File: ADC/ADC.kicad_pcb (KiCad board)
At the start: 2 copper layers, 38.1 x 63.5 mm, 98 parts, among them P1 CONN_02X05, P2 CONN_02X08, U1 MICA, U2 MICB, U3 TL074, U4 MICC, U5 MICD, U6 AK5703

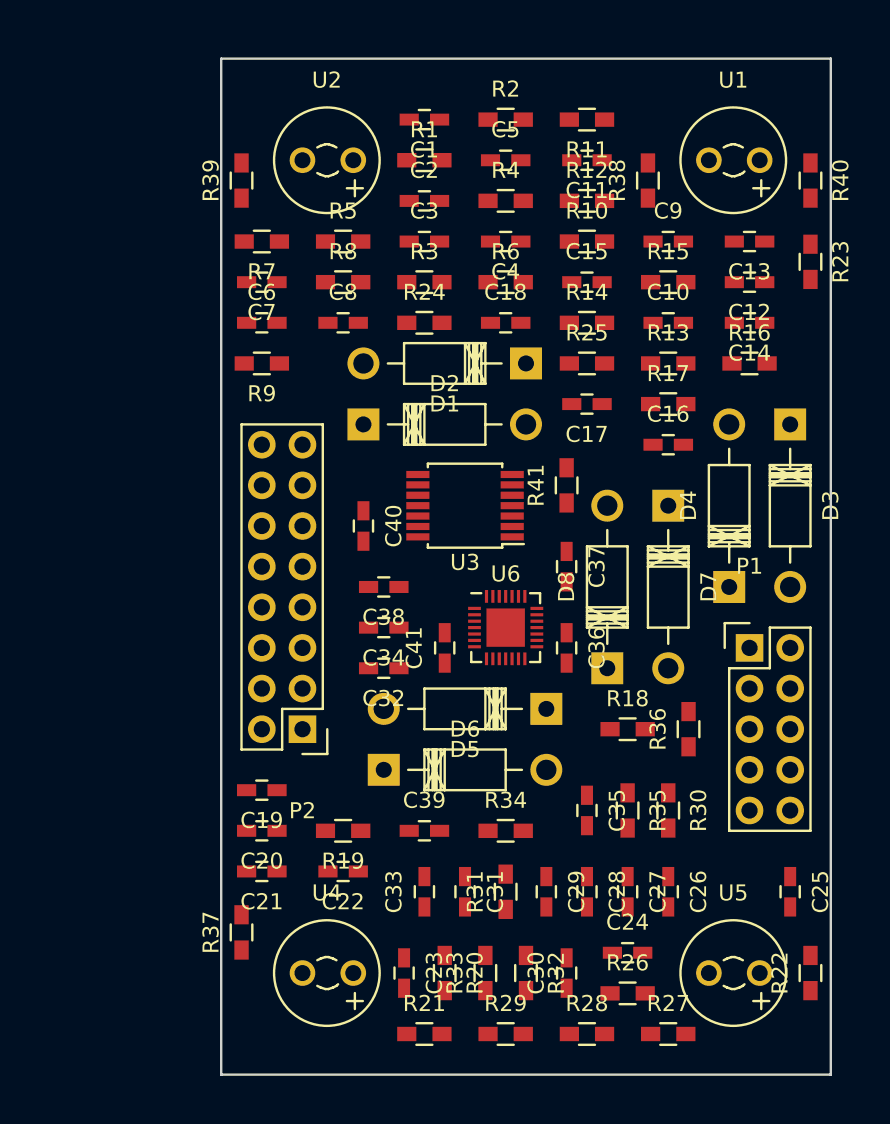
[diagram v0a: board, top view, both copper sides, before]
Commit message: Expanded board, all files
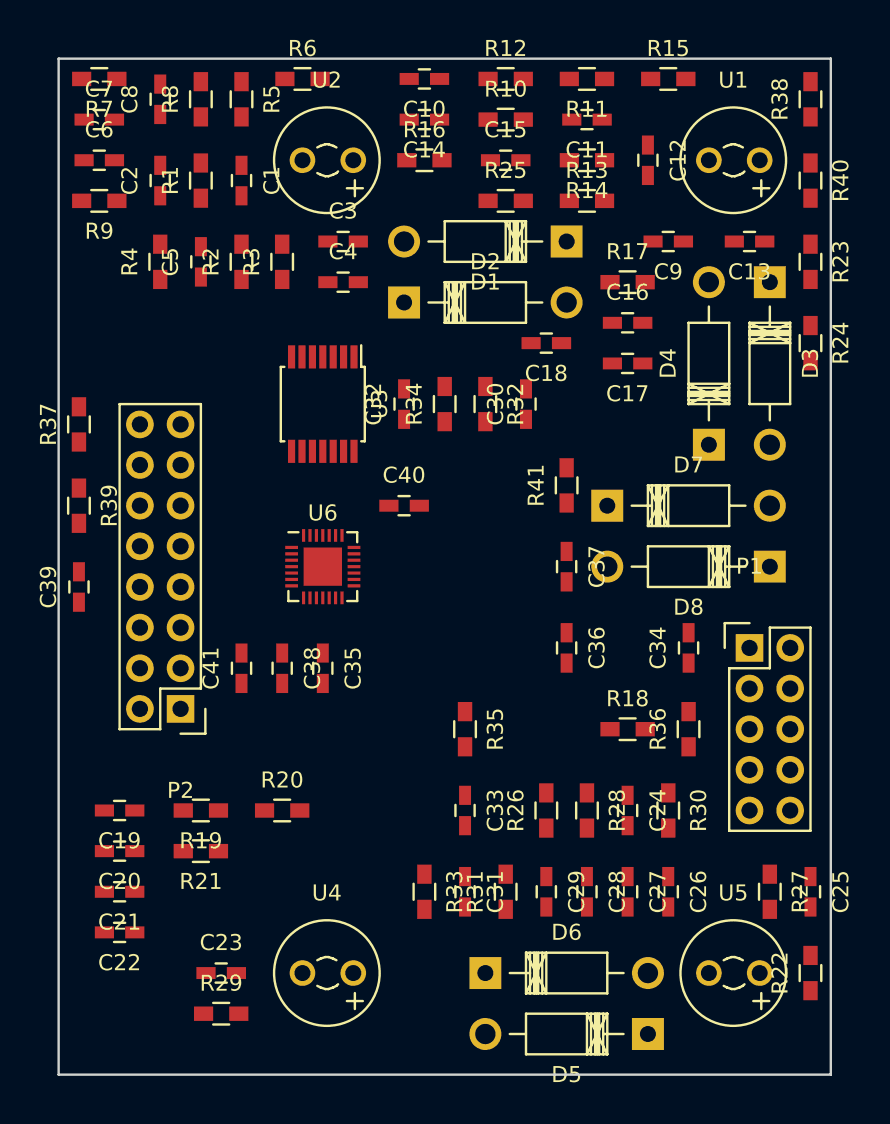
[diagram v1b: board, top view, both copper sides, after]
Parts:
- moved C30 35.7 mm to (94.0, 121.9)
- moved R32 35.7 mm to (91.4, 121.9)
- moved R37 33.3 mm to (66.0, 123.2)
- moved R34 26.9 mm to (88.9, 121.9), turned to 90 degrees
- moved C39 26.4 mm to (66.0, 133.3), turned to 90 degrees
- moved R24 24.2 mm to (111.8, 118.1), turned to 270 degrees
- moved C14 24.0 mm to (87.6, 104.1)
- moved R16 24.0 mm to (87.6, 106.7)
- moved R39 22.7 mm to (66.0, 128.3), turned to 270 degrees
- moved R4 21.9 mm to (71.1, 113.0), turned to 90 degrees
- moved C10 21.6 mm to (87.6, 101.6), turned to 180 degrees
- moved D5 21.3 mm to (96.5, 161.3)
- moved C5 20.1 mm to (73.7, 113.0), turned to 90 degrees
- moved C34 19.1 mm to (104.1, 137.2), turned to 90 degrees
- moved C35 18.8 mm to (81.3, 138.4)
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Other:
- board size 38.1 x 63.5 mm -> 48.3 x 63.5 mm
- net class Default: clearance 0.2 -> 0.1524; trace_width 0.25 -> 0.1524; via_dia 0.6 -> 0.3556; via_drill 0.4 -> 0.3302
- rule trace_clearance: 0.2 -> 0.1524
- rule trace_min: 0.2 -> 0.1524
- rule via_min_drill: 0.3 -> 0.3302
- rule via_min_size: 0.4 -> 0.3556
